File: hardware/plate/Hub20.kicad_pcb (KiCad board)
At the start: 4 copper layers, 89 x 124 mm, 4 parts

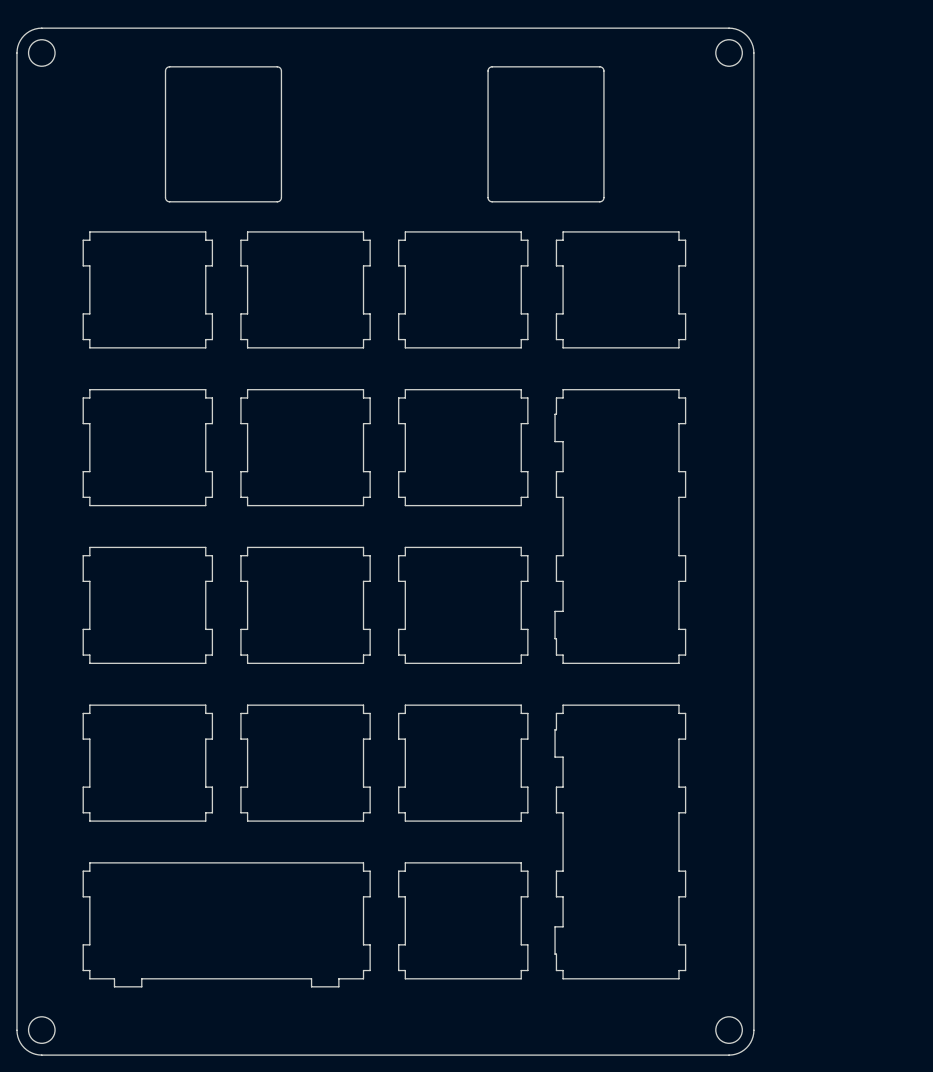
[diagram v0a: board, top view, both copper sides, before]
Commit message: stop touching the design josh
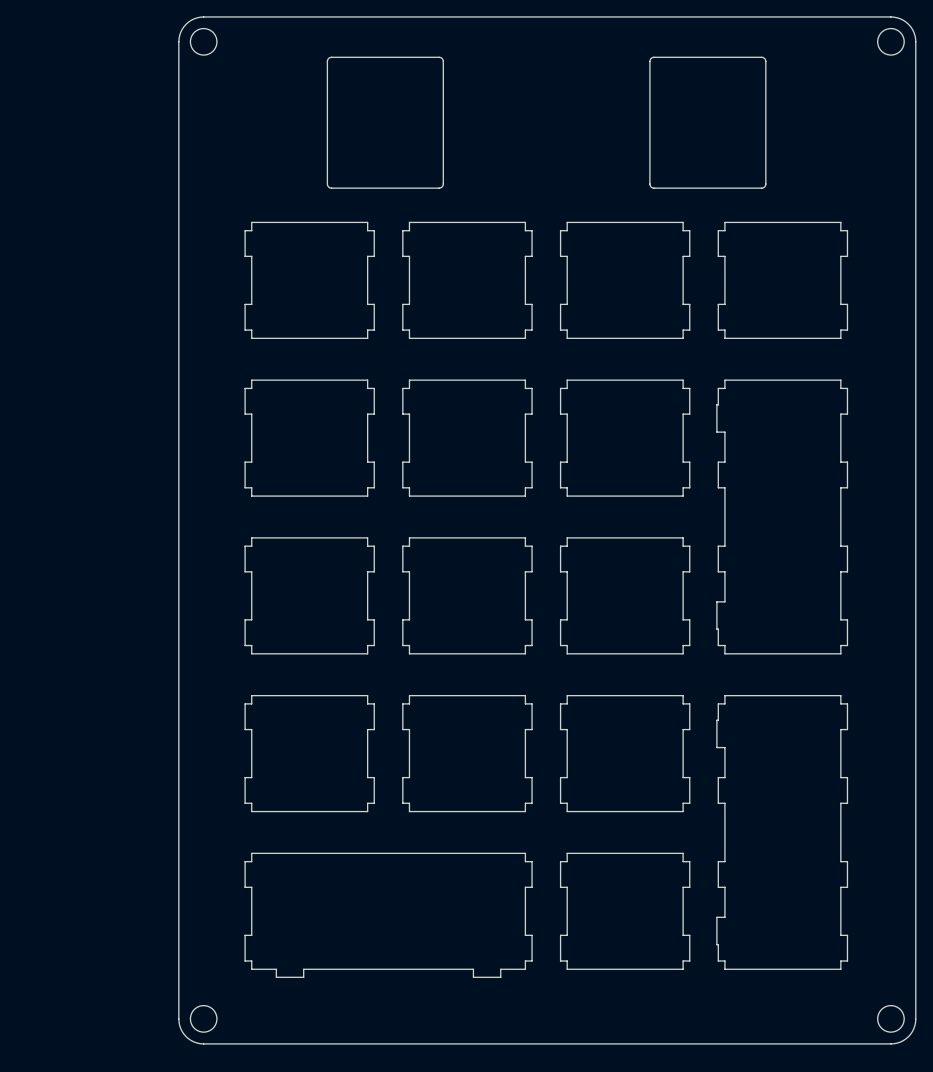
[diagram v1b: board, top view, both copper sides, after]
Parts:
- moved H2 19.6 mm to (97.5, 39.5)
- moved H4 19.6 mm to (97.5, 157.5)
- moved H1 19.6 mm to (180.4, 39.5)
- moved H3 19.6 mm to (180.4, 157.5)
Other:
- outline, holes or cut-outs redrawn
